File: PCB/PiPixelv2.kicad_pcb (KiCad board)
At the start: 2 copper layers, 65 x 30 mm, 13 parts, among them CON1 BARREL_JACK, J1 RPi_GPIO, P1 CONN_01X04, P2 CONN_01X02, U1 74AHC125

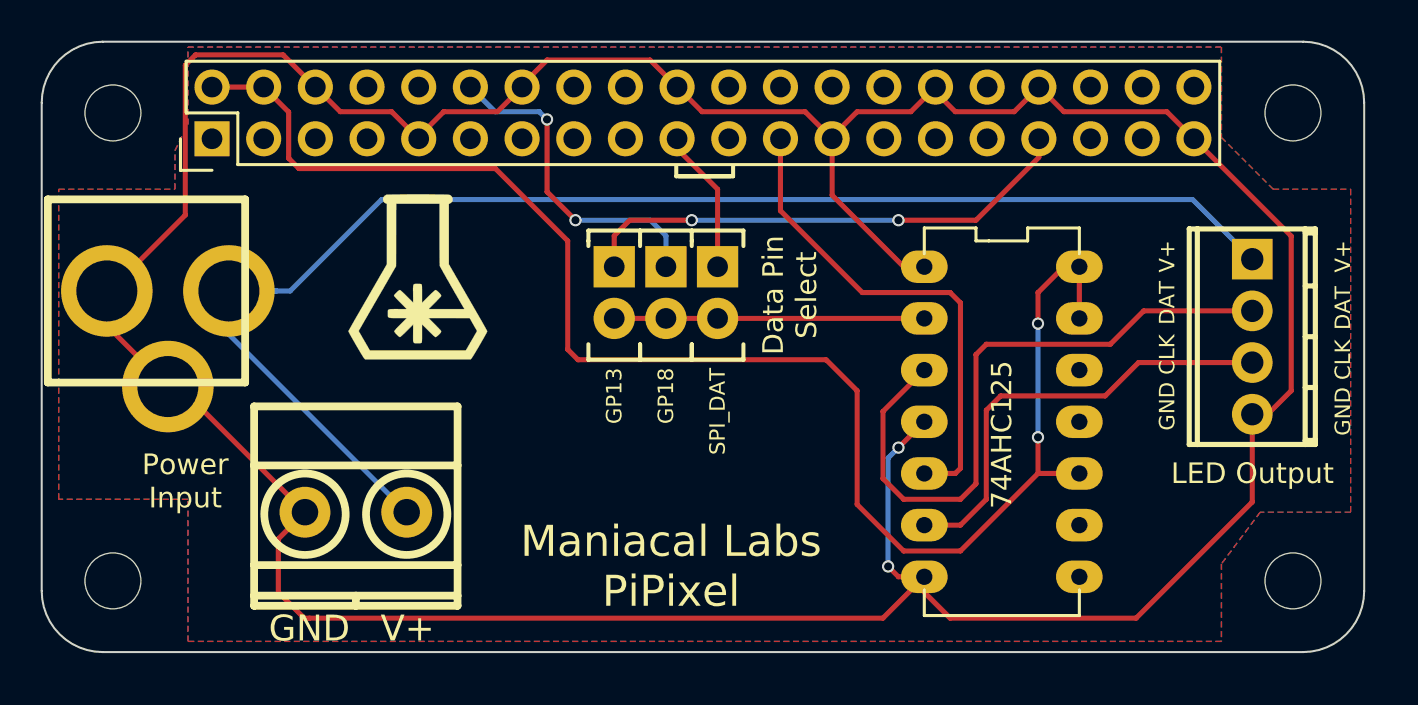
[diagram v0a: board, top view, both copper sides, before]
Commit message: Further PCB changes, library adds
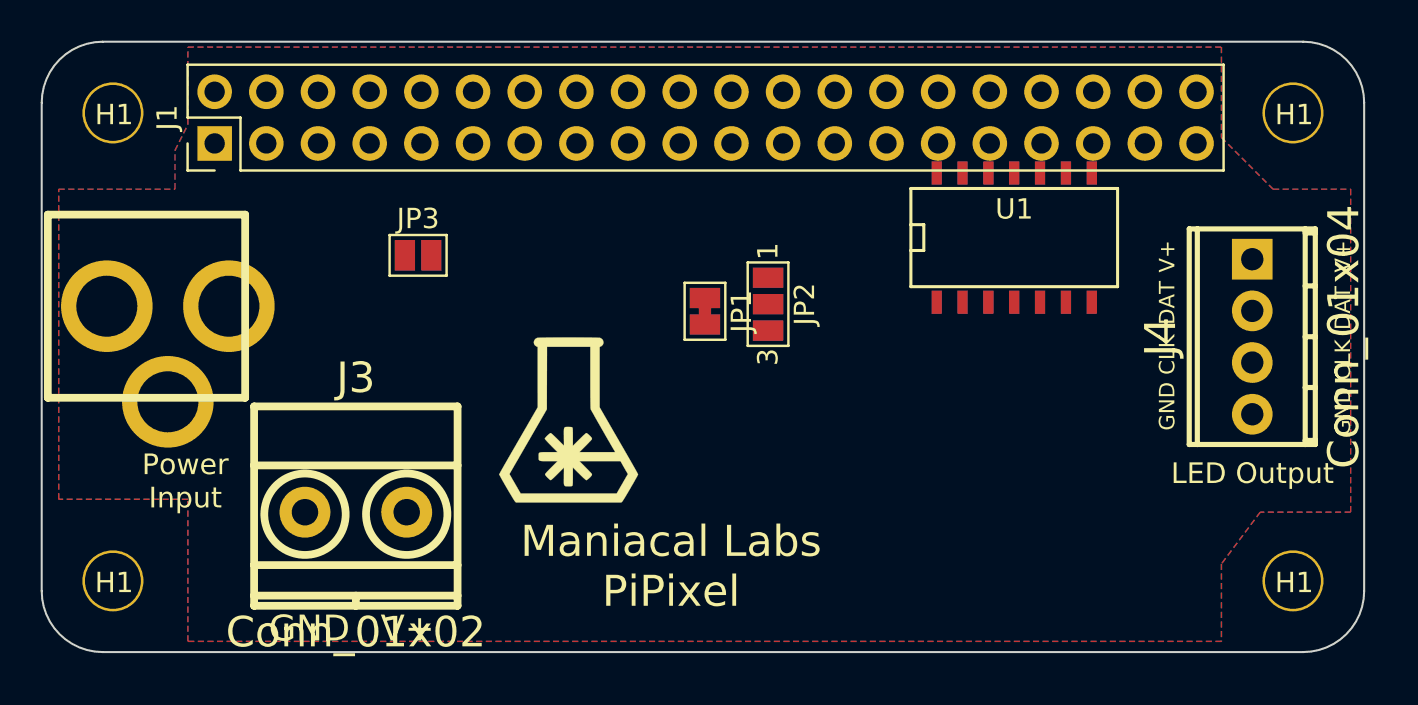
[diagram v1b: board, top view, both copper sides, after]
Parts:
- removed ? (x4): , RPi_Hat:RPi_Hat_Mounting_Hole
- removed CON1: BARREL_JACK, APM_BarrelJack:ML_BARREL_JACK_ROUND_PADS_SHORT
- removed P1: CONN_01X04, w_conn_mpt:mpt_0,5%2f4-2,54
- removed P2: CONN_01X02, w_conn_mkds:mkds_1,5-2
- added H1: 3mm_Mounting_Hole, RPi_HAT_MountingHole:NPTH_3mm_ID, F.Cu at (16.0, 28.0)
- added H1: 3mm_Mounting_Hole, RPi_HAT_MountingHole:NPTH_3mm_ID, F.Cu at (16.0, 51.0)
- added H1: 3mm_Mounting_Hole, RPi_HAT_MountingHole:NPTH_3mm_ID, F.Cu at (74.0, 51.0)
- added H1: 3mm_Mounting_Hole, RPi_HAT_MountingHole:NPTH_3mm_ID, F.Cu at (74.0, 28.0)
- added J2: Barrel_Jack_Switch, APM_BarrelJack:ML_BARREL_JACK_ROUND_PADS_SHORT, F.Cu at (15.5, 37.5)
- added J3: Conn_01x02, w_conn_mkds:mkds_1,5-2, F.Cu at (27.9, 47.6)
- added J4: Conn_01x04, w_conn_mpt:mpt_0,5%2f4-2,54, F.Cu at (72.0, 39.0)
- J1: value RPi_GPIO -> Raspberry_Pi_2_3; footprint RPi_Hat:Pin_Header_Straight_2x20 -> Pin_Headers:Pin_Header_Straight_2x20_Pitch2.54mm
- JP1: value Jumper_NC_Small -> SolderJumper_2_Bridged; footprint Custom:small_jump -> Jumper:SolderJumper-2_P1.3mm_Bridged_Pad1.0x1.5mm
- JP2: value Jumper_NO_Small -> SolderJumper_3_Open; footprint Custom:small_jump -> Jumper:SolderJumper-3_P1.3mm_Open_Pad1.0x1.5mm_NumberLabels
- JP3: value Jumper_NO_Small -> SolderJumper_2_Open; footprint Custom:small_jump -> Jumper:SolderJumper-2_P1.3mm_Open_Pad1.0x1.5mm
- U1: footprint Custom:DIP_14 -> SMD_Packages:SOIC-14_N
- moved J1 24.0 mm to (21.0, 29.5)
- moved G*** 10.2 mm to (38.4, 43.1)
- moved JP3 9.66 mm to (31.0, 35.0), turned to 0 degrees
- moved JP2 5.35 mm to (48.2, 37.4)
- moved U1 4.69 mm to (60.3, 34.0)
- moved JP1 2.28 mm to (45.1, 37.8)
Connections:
- JP1 pad 2: Net-(JP1-Pad2) -> LS_IN
- JP2 pad 2: Net-(JP1-Pad2) -> LS_IN
- JP3 pad 1: PWM_13 -> PWR
- JP3 pad 2: Net-(JP1-Pad2) -> 5V
- U1 pad 2: Net-(JP1-Pad2) -> LS_IN
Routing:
- net GND: track 183.2 -> 0.00 mm, vias 2 -> 0
- net 5V: track 75.4 -> 0.00 mm, vias 2 -> 0
- net PWR: track 70.2 -> 0.00 mm
- net Net-(J4-Pad2): track 32.3 -> 0.00 mm
- net PWM_13: track 24.9 -> 0.00 mm, vias 2 -> 0
- net CLK: track 24.3 -> 0.00 mm
- net Net-(J4-Pad3): track 22.0 -> 0.00 mm
- net PWM_18: track 16.2 -> 0.00 mm, vias 2 -> 0
- net Net-(JP1-Pad2): track 15.2 -> 0.00 mm
- net MOSI: track 7.11 -> 0.00 mm
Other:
- board text removed: "Data Pin Select"
- board text removed: "GP13"
- board text removed: "GP18"
- board text removed: "SPI_DAT"
